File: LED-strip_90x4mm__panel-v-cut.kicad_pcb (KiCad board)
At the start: 2 copper layers, 96 x 90 mm, 912 parts, among them P1 CONN_2, P10 CONN_2, P11 CONN_2, P12 CONN_2, P2 CONN_2, P3 CONN_2, P4 CONN_2, P5 CONN_2, P6 CONN_2, P7 CONN_2, P8 CONN_2, P9 CONN_2

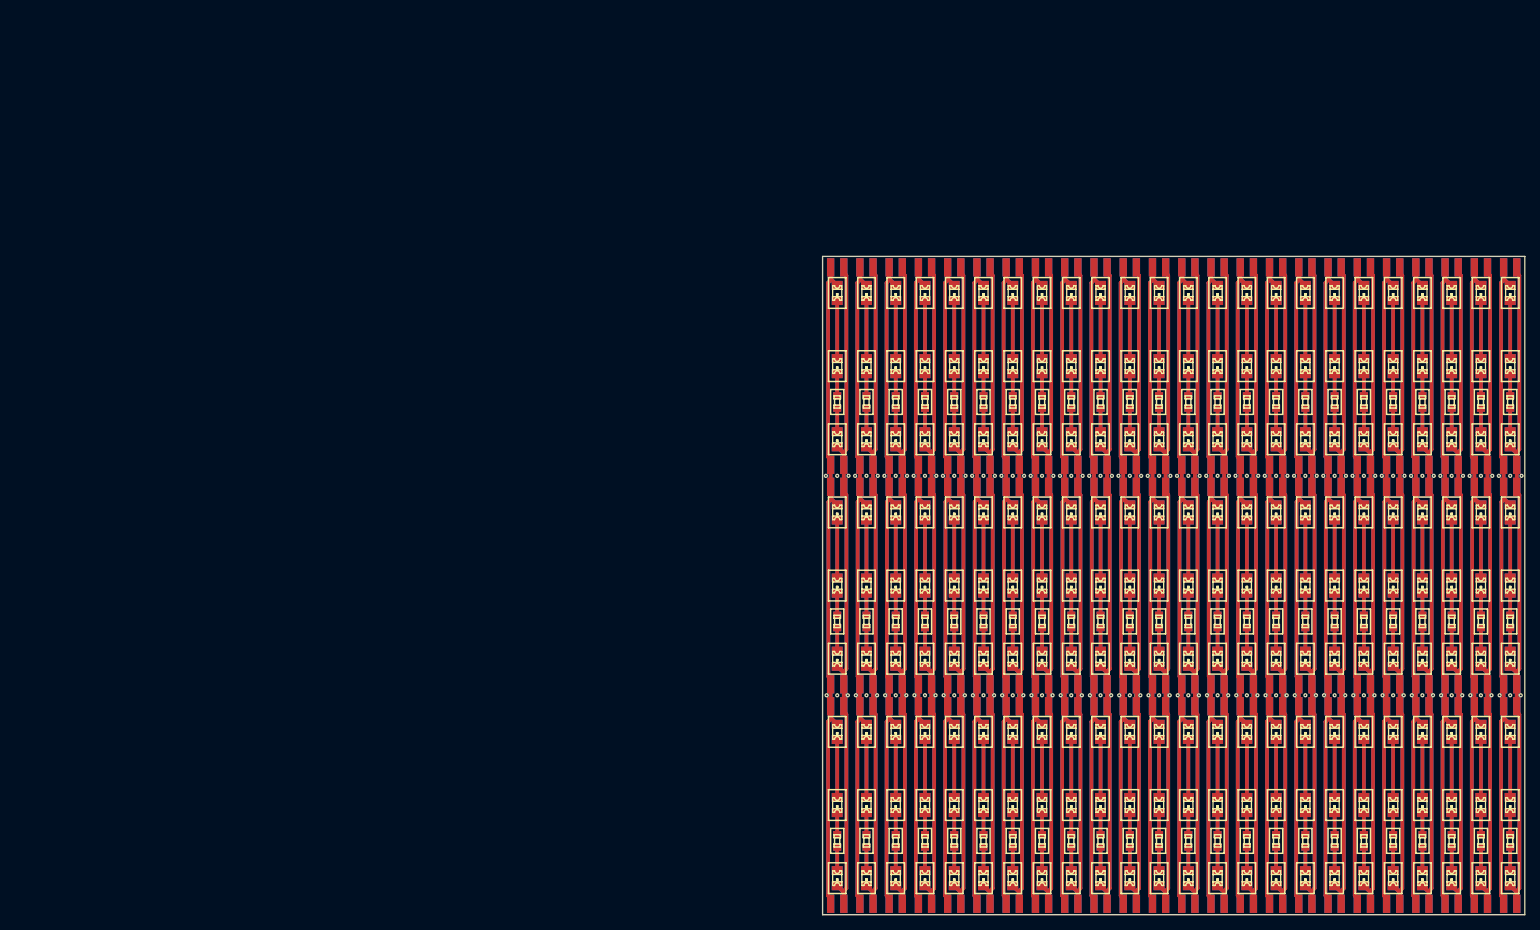
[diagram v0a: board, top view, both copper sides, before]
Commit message: Redid the panel.
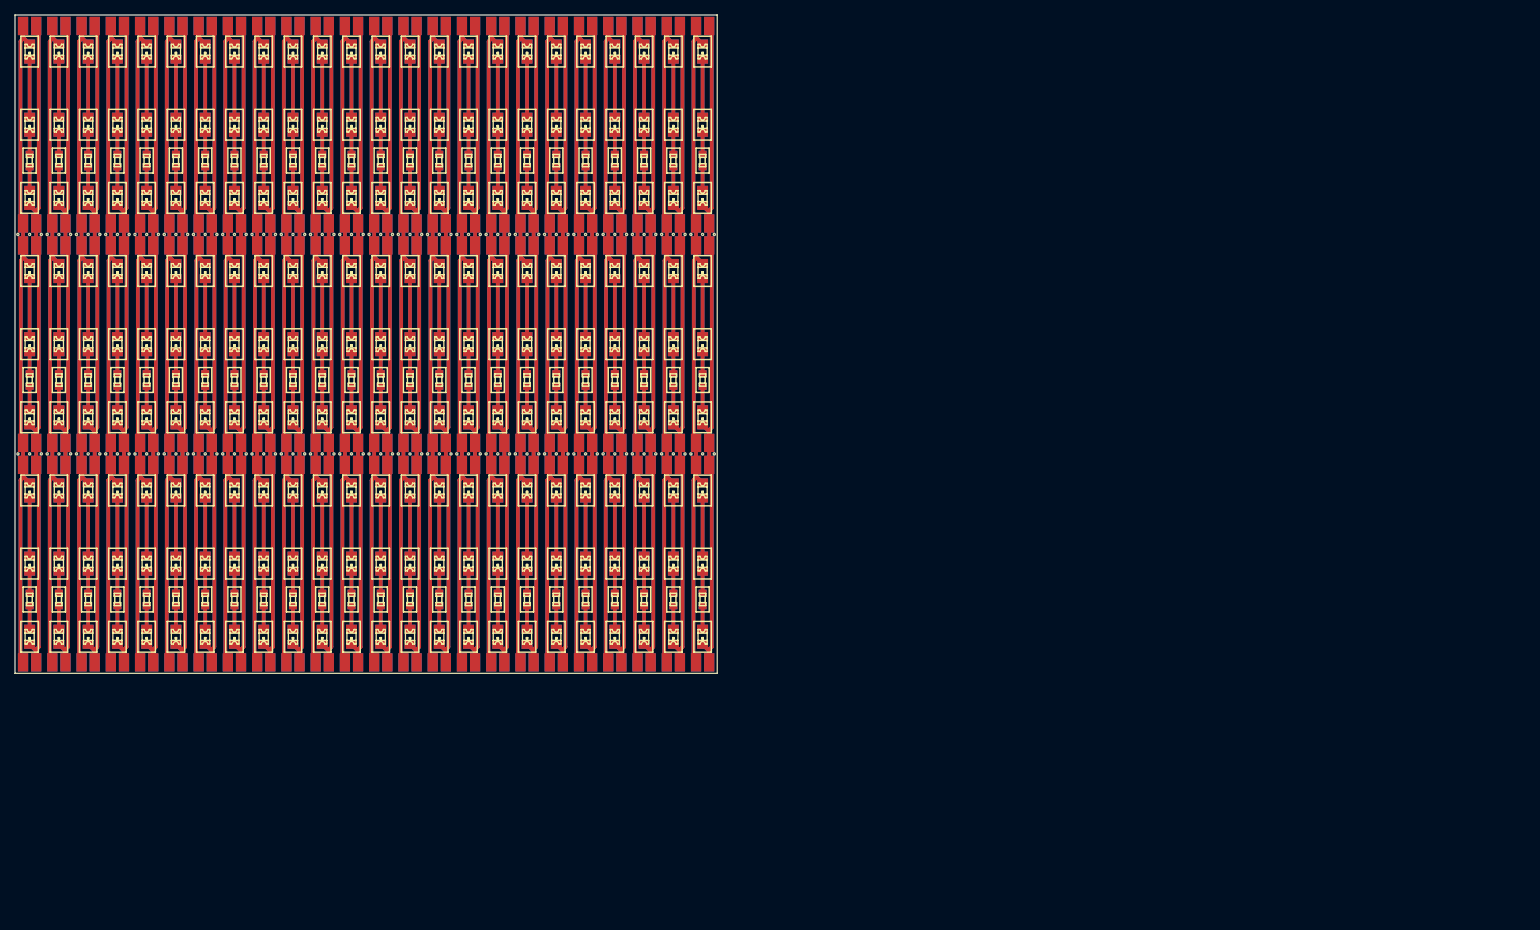
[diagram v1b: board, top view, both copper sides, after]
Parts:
- removed the D1 at (288.5, 153.0)
- removed the D1 at (328.5, 153.0)
- removed the D1 at (312.5, 153.0)
- removed the D1 at (316.5, 153.0)
- removed the D1 at (324.5, 153.0)
- removed the D1 at (320.5, 153.0)
- removed the D1 at (360.5, 153.0)
- removed the D1 at (364.5, 153.0)
- removed the D1 at (356.5, 153.0)
- removed the D1 at (352.5, 153.0)
- removed the D1 at (368.5, 153.0)
- removed the D1 at (284.5, 153.0)
- removed the D1 at (348.5, 153.0)
- removed the D1 at (332.5, 153.0)
- removed the D1 at (336.5, 153.0)
- removed the D1 at (344.5, 153.0)
- removed the D1 at (340.5, 153.0)
- removed the D1 at (372.5, 153.0)
- removed the D1 at (376.5, 153.0)
- removed the D1 at (300.5, 153.0)
- removed the D1 at (304.5, 153.0)
- removed the D1 at (296.5, 153.0)
- removed the D1 at (292.5, 153.0)
- removed the D1 at (308.5, 153.0)
- removed the D10 at (288.5, 93.0)
- removed the D10 at (328.5, 93.0)
- removed the D10 at (312.5, 93.0)
- removed the D10 at (316.5, 93.0)
- removed the D10 at (324.5, 93.0)
- removed the D10 at (320.5, 93.0)
- removed the D10 at (360.5, 93.0)
- removed the D10 at (364.5, 93.0)
- removed the D10 at (356.5, 93.0)
- removed the D10 at (352.5, 93.0)
- removed the D10 at (368.5, 93.0)
- removed the D10 at (284.5, 93.0)
- removed the D10 at (348.5, 93.0)
- removed the D10 at (332.5, 93.0)
- removed the D10 at (336.5, 93.0)
- removed the D10 at (344.5, 93.0)
- removed the D10 at (340.5, 93.0)
- removed the D10 at (372.5, 93.0)
- removed the D10 at (376.5, 93.0)
- removed the D10 at (300.5, 93.0)
- removed the D10 at (304.5, 93.0)
- removed the D10 at (296.5, 93.0)
- removed the D10 at (292.5, 93.0)
- removed the D10 at (308.5, 93.0)
- removed the D11 at (288.5, 103.0)
- removed the D11 at (328.5, 103.0)
- removed the D11 at (312.5, 103.0)
- removed the D11 at (316.5, 103.0)
- removed the D11 at (324.5, 103.0)
- removed the D11 at (320.5, 103.0)
- removed the D11 at (360.5, 103.0)
- removed the D11 at (364.5, 103.0)
- removed the D11 at (356.5, 103.0)
- removed the D11 at (352.5, 103.0)
- removed the D11 at (368.5, 103.0)
- removed the D11 at (284.5, 103.0)
- removed the D11 at (348.5, 103.0)
- removed the D11 at (332.5, 103.0)
- removed the D11 at (336.5, 103.0)
- removed the D11 at (344.5, 103.0)
- removed the D11 at (340.5, 103.0)
- removed the D11 at (372.5, 103.0)
- removed the D11 at (376.5, 103.0)
- removed the D11 at (300.5, 103.0)
- removed the D11 at (304.5, 103.0)
- removed the D11 at (296.5, 103.0)
- removed the D11 at (292.5, 103.0)
- removed the D11 at (308.5, 103.0)
- removed the D12 at (288.5, 113.0)
- removed the D12 at (328.5, 113.0)
- removed the D12 at (312.5, 113.0)
- removed the D12 at (316.5, 113.0)
- removed the D12 at (324.5, 113.0)
- removed the D12 at (320.5, 113.0)
- removed the D12 at (360.5, 113.0)
- removed the D12 at (364.5, 113.0)
- removed the D12 at (356.5, 113.0)
- removed the D12 at (352.5, 113.0)
- removed the D12 at (368.5, 113.0)
- removed the D12 at (284.5, 113.0)
- removed the D12 at (348.5, 113.0)
- removed the D12 at (332.5, 113.0)
- removed the D12 at (336.5, 113.0)
- removed the D12 at (344.5, 113.0)
- removed the D12 at (340.5, 113.0)
- removed the D12 at (372.5, 113.0)
- removed the D12 at (376.5, 113.0)
- removed the D12 at (300.5, 113.0)
- removed the D12 at (304.5, 113.0)
- removed the D12 at (296.5, 113.0)
- removed the D12 at (292.5, 113.0)
- removed the D12 at (308.5, 113.0)
- removed the D13 at (288.5, 123.0)
- removed the D13 at (328.5, 123.0)
- removed the D13 at (312.5, 123.0)
- removed the D13 at (316.5, 123.0)
- removed the D13 at (324.5, 123.0)
- removed the D13 at (320.5, 123.0)
- removed the D13 at (360.5, 123.0)
- removed the D13 at (364.5, 123.0)
- removed the D13 at (356.5, 123.0)
- removed the D13 at (352.5, 123.0)
- removed the D13 at (368.5, 123.0)
- removed the D13 at (284.5, 123.0)
- removed the D13 at (348.5, 123.0)
- removed the D13 at (332.5, 123.0)
- removed the D13 at (336.5, 123.0)
- removed the D13 at (344.5, 123.0)
- removed the D13 at (340.5, 123.0)
- removed the D13 at (372.5, 123.0)
- removed the D13 at (376.5, 123.0)
- removed the D13 at (300.5, 123.0)
- removed the D13 at (304.5, 123.0)
- removed the D13 at (296.5, 123.0)
- removed the D13 at (292.5, 123.0)
- removed the D13 at (308.5, 123.0)
- removed the D14 at (288.5, 133.0)
- removed the D14 at (328.5, 133.0)
- removed the D14 at (312.5, 133.0)
- removed the D14 at (316.5, 133.0)
- removed the D14 at (324.5, 133.0)
- removed the D14 at (320.5, 133.0)
- removed the D14 at (360.5, 133.0)
- removed the D14 at (364.5, 133.0)
- removed the D14 at (356.5, 133.0)
- removed the D14 at (352.5, 133.0)
- removed the D14 at (368.5, 133.0)
- removed the D14 at (284.5, 133.0)
- removed the D14 at (348.5, 133.0)
- removed the D14 at (332.5, 133.0)
- removed the D14 at (336.5, 133.0)
- removed the D14 at (344.5, 133.0)
- removed the D14 at (340.5, 133.0)
- removed the D14 at (372.5, 133.0)
- removed the D14 at (376.5, 133.0)
- removed the D14 at (300.5, 133.0)
- removed the D14 at (304.5, 133.0)
- removed the D14 at (296.5, 133.0)
- removed the D14 at (292.5, 133.0)
- removed the D14 at (308.5, 133.0)
- removed the D15 at (288.5, 143.0)
- removed the D15 at (328.5, 143.0)
- removed the D15 at (312.5, 143.0)
- removed the D15 at (316.5, 143.0)
- removed the D15 at (324.5, 143.0)
- removed the D15 at (320.5, 143.0)
- removed the D15 at (360.5, 143.0)
- removed the D15 at (364.5, 143.0)
- removed the D15 at (356.5, 143.0)
- removed the D15 at (352.5, 143.0)
- removed the D15 at (368.5, 143.0)
- removed the D15 at (284.5, 143.0)
- removed the D15 at (348.5, 143.0)
- removed the D15 at (332.5, 143.0)
- removed the D15 at (336.5, 143.0)
- removed the D15 at (344.5, 143.0)
- removed the D15 at (340.5, 143.0)
- removed the D15 at (372.5, 143.0)
- removed the D15 at (376.5, 143.0)
- removed the D15 at (300.5, 143.0)
- removed the D15 at (304.5, 143.0)
- removed the D15 at (296.5, 143.0)
- removed the D15 at (292.5, 143.0)
- removed the D15 at (308.5, 143.0)
- removed the D16 at (288.5, 153.0)
- removed the D16 at (328.5, 153.0)
- removed the D16 at (312.5, 153.0)
- removed the D16 at (316.5, 153.0)
- removed the D16 at (324.5, 153.0)
- removed the D16 at (320.5, 153.0)
- removed the D16 at (360.5, 153.0)
- removed the D16 at (364.5, 153.0)
- removed the D16 at (356.5, 153.0)
- removed the D16 at (352.5, 153.0)
- removed the D16 at (368.5, 153.0)
- removed the D16 at (284.5, 153.0)
- removed the D16 at (348.5, 153.0)
- removed the D16 at (332.5, 153.0)
- removed the D16 at (336.5, 153.0)
- removed the D16 at (344.5, 153.0)
- removed the D16 at (340.5, 153.0)
- removed the D16 at (372.5, 153.0)
- removed the D16 at (376.5, 153.0)
- removed the D16 at (300.5, 153.0)
- removed the D16 at (304.5, 153.0)
- removed the D16 at (296.5, 153.0)
- removed the D16 at (292.5, 153.0)
- removed the D16 at (308.5, 153.0)
- removed the D17 at (288.5, 163.0)
- removed the D17 at (328.5, 163.0)
- removed the D17 at (312.5, 163.0)
- removed the D17 at (316.5, 163.0)
- removed the D17 at (324.5, 163.0)
- removed the D17 at (320.5, 163.0)
- removed the D17 at (360.5, 163.0)
- removed the D17 at (364.5, 163.0)
- removed the D17 at (356.5, 163.0)
- removed the D17 at (352.5, 163.0)
- removed the D17 at (368.5, 163.0)
- removed the D17 at (284.5, 163.0)
- removed the D17 at (348.5, 163.0)
- removed the D17 at (332.5, 163.0)
- removed the D17 at (336.5, 163.0)
- removed the D17 at (344.5, 163.0)
- removed the D17 at (340.5, 163.0)
- removed the D17 at (372.5, 163.0)
- removed the D17 at (376.5, 163.0)
- removed the D17 at (300.5, 163.0)
- removed the D17 at (304.5, 163.0)
- removed the D17 at (296.5, 163.0)
- removed the D17 at (292.5, 163.0)
- removed the D17 at (308.5, 163.0)
- removed the D18 at (288.5, 173.0)
- removed the D18 at (328.5, 173.0)
- removed the D18 at (312.5, 173.0)
- removed the D18 at (316.5, 173.0)
- removed the D18 at (324.5, 173.0)
- removed the D18 at (320.5, 173.0)
- removed the D18 at (360.5, 173.0)
- removed the D18 at (364.5, 173.0)
- removed the D18 at (356.5, 173.0)
- removed the D18 at (352.5, 173.0)
- removed the D18 at (368.5, 173.0)
- removed the D18 at (284.5, 173.0)
- removed the D18 at (348.5, 173.0)
- removed the D18 at (332.5, 173.0)
- removed the D18 at (336.5, 173.0)
- removed the D18 at (344.5, 173.0)
- removed the D18 at (340.5, 173.0)
- removed the D18 at (372.5, 173.0)
- removed the D18 at (376.5, 173.0)
- removed the D18 at (300.5, 173.0)
- removed the D18 at (304.5, 173.0)
- removed the D18 at (296.5, 173.0)
- removed the D18 at (292.5, 173.0)
- removed the D18 at (308.5, 173.0)
- removed the D2 at (288.5, 163.0)
- removed the D2 at (328.5, 163.0)
- removed the D2 at (312.5, 163.0)
- removed the D2 at (316.5, 163.0)
- removed the D2 at (324.5, 163.0)
- removed the D2 at (320.5, 163.0)
- removed the D2 at (360.5, 163.0)
- removed the D2 at (364.5, 163.0)
- removed the D2 at (356.5, 163.0)
- removed the D2 at (352.5, 163.0)
- removed the D2 at (368.5, 163.0)
- removed the D2 at (284.5, 163.0)
- removed the D2 at (348.5, 163.0)
- removed the D2 at (332.5, 163.0)
- removed the D2 at (336.5, 163.0)
- removed the D2 at (344.5, 163.0)
- removed the D2 at (340.5, 163.0)
- removed the D2 at (372.5, 163.0)
- removed the D2 at (376.5, 163.0)
- removed the D2 at (300.5, 163.0)
- removed the D2 at (304.5, 163.0)
- removed the D2 at (296.5, 163.0)
- removed the D2 at (292.5, 163.0)
- removed the D2 at (308.5, 163.0)
- removed the D3 at (288.5, 173.0)
- removed the D3 at (328.5, 173.0)
- removed the D3 at (312.5, 173.0)
- removed the D3 at (316.5, 173.0)
- removed the D3 at (324.5, 173.0)
- removed the D3 at (320.5, 173.0)
- removed the D3 at (360.5, 173.0)
- removed the D3 at (364.5, 173.0)
- removed the D3 at (356.5, 173.0)
- removed the D3 at (352.5, 173.0)
- removed the D3 at (368.5, 173.0)
- removed the D3 at (284.5, 173.0)
- removed the D3 at (348.5, 173.0)
- removed the D3 at (332.5, 173.0)
- removed the D3 at (336.5, 173.0)
- removed the D3 at (344.5, 173.0)
- removed the D3 at (340.5, 173.0)
- removed the D3 at (372.5, 173.0)
- removed the D3 at (376.5, 173.0)
- removed the D3 at (300.5, 173.0)
- removed the D3 at (304.5, 173.0)
- removed the D3 at (296.5, 173.0)
- removed the D3 at (292.5, 173.0)
- removed the D3 at (308.5, 173.0)
- removed the D4 at (288.5, 123.0)
- removed the D4 at (328.5, 123.0)
- removed the D4 at (312.5, 123.0)
- removed the D4 at (316.5, 123.0)
- removed the D4 at (324.5, 123.0)
- removed the D4 at (320.5, 123.0)
- removed the D4 at (360.5, 123.0)
- removed the D4 at (364.5, 123.0)
- removed the D4 at (356.5, 123.0)
- removed the D4 at (352.5, 123.0)
- removed the D4 at (368.5, 123.0)
- removed the D4 at (284.5, 123.0)
- removed the D4 at (348.5, 123.0)
- removed the D4 at (332.5, 123.0)
- removed the D4 at (336.5, 123.0)
- removed the D4 at (344.5, 123.0)
- removed the D4 at (340.5, 123.0)
- removed the D4 at (372.5, 123.0)
- removed the D4 at (376.5, 123.0)
- removed the D4 at (300.5, 123.0)
- removed the D4 at (304.5, 123.0)
- removed the D4 at (296.5, 123.0)
- removed the D4 at (292.5, 123.0)
- removed the D4 at (308.5, 123.0)
- removed the D5 at (288.5, 133.0)
- removed the D5 at (328.5, 133.0)
- removed the D5 at (312.5, 133.0)
- removed the D5 at (316.5, 133.0)
- removed the D5 at (324.5, 133.0)
- removed the D5 at (320.5, 133.0)
- removed the D5 at (360.5, 133.0)
- removed the D5 at (364.5, 133.0)
- removed the D5 at (356.5, 133.0)
- removed the D5 at (352.5, 133.0)
- removed the D5 at (368.5, 133.0)
- removed the D5 at (284.5, 133.0)
- removed the D5 at (348.5, 133.0)
- removed the D5 at (332.5, 133.0)
- removed the D5 at (336.5, 133.0)
- removed the D5 at (344.5, 133.0)
- removed the D5 at (340.5, 133.0)
- removed the D5 at (372.5, 133.0)
- removed the D5 at (376.5, 133.0)
- removed the D5 at (300.5, 133.0)
- removed the D5 at (304.5, 133.0)
- removed the D5 at (296.5, 133.0)
- removed the D5 at (292.5, 133.0)
- removed the D5 at (308.5, 133.0)
- removed the D6 at (288.5, 143.0)
- removed the D6 at (328.5, 143.0)
- removed the D6 at (312.5, 143.0)
- removed the D6 at (316.5, 143.0)
- removed the D6 at (324.5, 143.0)
- removed the D6 at (320.5, 143.0)
- removed the D6 at (360.5, 143.0)
- removed the D6 at (364.5, 143.0)
- removed the D6 at (356.5, 143.0)
- removed the D6 at (352.5, 143.0)
- removed the D6 at (368.5, 143.0)
- removed the D6 at (284.5, 143.0)
- removed the D6 at (348.5, 143.0)
- removed the D6 at (332.5, 143.0)
- removed the D6 at (336.5, 143.0)
- removed the D6 at (344.5, 143.0)
- removed the D6 at (340.5, 143.0)
- removed the D6 at (372.5, 143.0)
- removed the D6 at (376.5, 143.0)
- removed the D6 at (300.5, 143.0)
- removed the D6 at (304.5, 143.0)
- removed the D6 at (296.5, 143.0)
- removed the D6 at (292.5, 143.0)
- removed the D6 at (308.5, 143.0)
- removed the D7 at (288.5, 93.0)
- removed the D7 at (328.5, 93.0)
- removed the D7 at (312.5, 93.0)
- removed the D7 at (316.5, 93.0)
- removed the D7 at (324.5, 93.0)
- removed the D7 at (320.5, 93.0)
- removed the D7 at (360.5, 93.0)
- removed the D7 at (364.5, 93.0)
- removed the D7 at (356.5, 93.0)
- removed the D7 at (352.5, 93.0)
- removed the D7 at (368.5, 93.0)
- removed the D7 at (284.5, 93.0)
- removed the D7 at (348.5, 93.0)
- removed the D7 at (332.5, 93.0)
- removed the D7 at (336.5, 93.0)
- removed the D7 at (344.5, 93.0)
- removed the D7 at (340.5, 93.0)
- removed the D7 at (372.5, 93.0)
- removed the D7 at (376.5, 93.0)
- removed the D7 at (300.5, 93.0)
- removed the D7 at (304.5, 93.0)
- removed the D7 at (296.5, 93.0)
- removed the D7 at (292.5, 93.0)
- removed the D7 at (308.5, 93.0)
- removed the D8 at (288.5, 103.0)
- removed the D8 at (328.5, 103.0)
- removed the D8 at (312.5, 103.0)
- removed the D8 at (316.5, 103.0)
- removed the D8 at (324.5, 103.0)
- removed the D8 at (320.5, 103.0)
- removed the D8 at (360.5, 103.0)
- removed the D8 at (364.5, 103.0)
- removed the D8 at (356.5, 103.0)
- removed the D8 at (352.5, 103.0)
- removed the D8 at (368.5, 103.0)
- removed the D8 at (284.5, 103.0)
- removed the D8 at (348.5, 103.0)
- removed the D8 at (332.5, 103.0)
- removed the D8 at (336.5, 103.0)
- removed the D8 at (344.5, 103.0)
- removed the D8 at (340.5, 103.0)
- removed the D8 at (372.5, 103.0)
- removed the D8 at (376.5, 103.0)
- removed the D8 at (300.5, 103.0)
- removed the D8 at (304.5, 103.0)
- removed the D8 at (296.5, 103.0)
- removed the D8 at (292.5, 103.0)
- removed the D8 at (308.5, 103.0)
- removed the D9 at (288.5, 113.0)
- removed the D9 at (328.5, 113.0)
- removed the D9 at (312.5, 113.0)
- removed the D9 at (316.5, 113.0)
- removed the D9 at (324.5, 113.0)
- removed the D9 at (320.5, 113.0)
- removed the D9 at (360.5, 113.0)
- removed the D9 at (364.5, 113.0)
- removed the D9 at (356.5, 113.0)
- removed the D9 at (352.5, 113.0)
- removed the D9 at (368.5, 113.0)
- removed the D9 at (284.5, 113.0)
- removed the D9 at (348.5, 113.0)
- removed the D9 at (332.5, 113.0)
- removed the D9 at (336.5, 113.0)
- removed the D9 at (344.5, 113.0)
- removed the D9 at (340.5, 113.0)
- removed the D9 at (372.5, 113.0)
- removed the D9 at (376.5, 113.0)
- removed the D9 at (300.5, 113.0)
- removed the D9 at (304.5, 113.0)
- removed the D9 at (296.5, 113.0)
- removed the D9 at (292.5, 113.0)
- removed the D9 at (308.5, 113.0)
- removed the G1 at (288.6, 98.1)
- removed the G1 at (328.6, 98.1)
- removed the G1 at (312.6, 98.1)
- removed the G1 at (316.6, 98.1)
- removed the G1 at (324.6, 98.1)
- removed the G1 at (320.6, 98.1)
- removed the G1 at (360.6, 98.1)
- removed the G1 at (364.6, 98.1)
- removed the G1 at (356.6, 98.1)
- removed the G1 at (352.6, 98.1)
- removed the G1 at (368.6, 98.1)
- removed the G1 at (284.6, 98.1)
- removed the G1 at (348.6, 98.1)
- removed the G1 at (332.6, 98.1)
- removed the G1 at (336.6, 98.1)
- removed the G1 at (344.6, 98.1)
- removed the G1 at (340.6, 98.1)
- removed the G1 at (372.6, 98.1)
- removed the G1 at (376.6, 98.1)
- removed the G1 at (300.6, 98.1)
- removed the G1 at (304.6, 98.1)
- removed the G1 at (296.6, 98.1)
- removed the G1 at (292.6, 98.1)
- removed the G1 at (308.6, 98.1)
- removed the G2 at (288.5, 128.1)
- removed the G2 at (328.5, 128.1)
- removed the G2 at (312.5, 128.1)
- removed the G2 at (316.5, 128.1)
- removed the G2 at (324.5, 128.1)
- removed the G2 at (320.5, 128.1)
- removed the G2 at (360.5, 128.1)
- removed the G2 at (364.5, 128.1)
- removed the G2 at (356.5, 128.1)
- removed the G2 at (352.5, 128.1)
- removed the G2 at (368.5, 128.1)
- removed the G2 at (284.5, 128.1)
- removed the G2 at (348.5, 128.1)
- removed the G2 at (332.5, 128.1)
- removed the G2 at (336.5, 128.1)
- removed the G2 at (344.5, 128.1)
- removed the G2 at (340.5, 128.1)
- removed the G2 at (372.5, 128.1)
- removed the G2 at (376.5, 128.1)
- removed the G2 at (300.5, 128.1)
- removed the G2 at (304.5, 128.1)
- removed the G2 at (296.5, 128.1)
- removed the G2 at (292.5, 128.1)
- removed the G2 at (308.5, 128.1)
- removed the P1 at (288.5, 176.5)
- removed the P1 at (328.5, 176.5)
- removed the P1 at (312.5, 176.5)
- removed the P1 at (316.5, 176.5)
- removed the P1 at (324.5, 176.5)
- removed the P1 at (320.5, 176.5)
- removed the P1 at (360.5, 176.5)
- removed the P1 at (364.5, 176.5)
- removed the P1 at (356.5, 176.5)
- removed the P1 at (352.5, 176.5)
- removed the P1 at (368.5, 176.5)
- removed the P1 at (284.5, 176.5)
- removed the P1 at (348.5, 176.5)
- removed the P1 at (332.5, 176.5)
- removed the P1 at (336.5, 176.5)
- removed the P1 at (344.5, 176.5)
- removed the P1 at (340.5, 176.5)
- removed the P1 at (372.5, 176.5)
- removed the P1 at (376.5, 176.5)
- removed the P1 at (300.5, 176.5)
- removed the P1 at (304.5, 176.5)
- removed the P1 at (296.5, 176.5)
- removed the P1 at (292.5, 176.5)
- removed the P1 at (308.5, 176.5)
- removed the P10 at (288.5, 146.5)
- removed the P10 at (328.5, 146.5)
- removed the P10 at (312.5, 146.5)
- removed the P10 at (316.5, 146.5)
- removed the P10 at (324.5, 146.5)
- removed the P10 at (320.5, 146.5)
- removed the P10 at (360.5, 146.5)
- removed the P10 at (364.5, 146.5)
- removed the P10 at (356.5, 146.5)
- removed the P10 at (352.5, 146.5)
- removed the P10 at (368.5, 146.5)
- removed the P10 at (284.5, 146.5)
- removed the P10 at (348.5, 146.5)
- removed the P10 at (332.5, 146.5)
- removed the P10 at (336.5, 146.5)
- removed the P10 at (344.5, 146.5)
- removed the P10 at (340.5, 146.5)
- removed the P10 at (372.5, 146.5)
- removed the P10 at (376.5, 146.5)
- removed the P10 at (300.5, 146.5)
- removed the P10 at (304.5, 146.5)
- removed the P10 at (296.5, 146.5)
- removed the P10 at (292.5, 146.5)
- removed the P10 at (308.5, 146.5)
- removed the P11 at (288.5, 149.5)
- removed the P11 at (328.5, 149.5)
- removed the P11 at (312.5, 149.5)
- removed the P11 at (316.5, 149.5)
- removed the P11 at (324.5, 149.5)
- removed the P11 at (320.5, 149.5)
- removed the P11 at (360.5, 149.5)
- removed the P11 at (364.5, 149.5)
- removed the P11 at (356.5, 149.5)
- removed the P11 at (352.5, 149.5)
- removed the P11 at (368.5, 149.5)
- removed the P11 at (284.5, 149.5)
- removed the P11 at (348.5, 149.5)
- removed the P11 at (332.5, 149.5)
- removed the P11 at (336.5, 149.5)
- removed the P11 at (344.5, 149.5)
- removed the P11 at (340.5, 149.5)
- removed the P11 at (372.5, 149.5)
- removed the P11 at (376.5, 149.5)
- removed the P11 at (300.5, 149.5)
- removed the P11 at (304.5, 149.5)
- removed the P11 at (296.5, 149.5)
- removed the P11 at (292.5, 149.5)
- removed the P11 at (308.5, 149.5)
- removed the P12 at (288.5, 176.5)
- removed the P12 at (328.5, 176.5)
- removed the P12 at (312.5, 176.5)
- removed the P12 at (316.5, 176.5)
- removed the P12 at (324.5, 176.5)
- removed the P12 at (320.5, 176.5)
- removed the P12 at (360.5, 176.5)
- removed the P12 at (364.5, 176.5)
- removed the P12 at (356.5, 176.5)
- removed the P12 at (352.5, 176.5)
- removed the P12 at (368.5, 176.5)
- removed the P12 at (284.5, 176.5)
- removed the P12 at (348.5, 176.5)
- removed the P12 at (332.5, 176.5)
- removed the P12 at (336.5, 176.5)
- removed the P12 at (344.5, 176.5)
- removed the P12 at (340.5, 176.5)
- removed the P12 at (372.5, 176.5)
- removed the P12 at (376.5, 176.5)
- removed the P12 at (300.5, 176.5)
- removed the P12 at (304.5, 176.5)
- removed the P12 at (296.5, 176.5)
- removed the P12 at (292.5, 176.5)
- removed the P12 at (308.5, 176.5)
- removed the P2 at (288.5, 149.5)
- removed the P2 at (348.5, 149.5)
- removed the P2 at (344.5, 149.5)
- removed the P2 at (340.5, 149.5)
- removed the P2 at (336.5, 149.5)
- removed the P2 at (332.5, 149.5)
- removed the P2 at (328.5, 149.5)
- removed the P2 at (324.5, 149.5)
- removed the P2 at (320.5, 149.5)
- removed the P2 at (316.5, 149.5)
- removed the P2 at (312.5, 149.5)
- removed the P2 at (284.5, 149.5)
- removed the P2 at (308.5, 149.5)
- removed the P2 at (304.5, 149.5)
- removed the P2 at (300.5, 149.5)
- removed the P2 at (296.5, 149.5)
- removed the P2 at (292.5, 149.5)
- removed the P2 at (372.5, 149.5)
- removed the P2 at (376.5, 149.5)
- removed the P2 at (368.5, 149.5)
- removed the P2 at (364.5, 149.5)
- removed the P2 at (360.5, 149.5)
- removed the P2 at (356.5, 149.5)
- removed the P2 at (352.5, 149.5)
- removed the P3 at (288.5, 146.5)
- removed the P3 at (328.5, 146.5)
- removed the P3 at (312.5, 146.5)
- removed the P3 at (316.5, 146.5)
- removed the P3 at (324.5, 146.5)
- removed the P3 at (320.5, 146.5)
- removed the P3 at (360.5, 146.5)
- removed the P3 at (364.5, 146.5)
- removed the P3 at (356.5, 146.5)
- removed the P3 at (352.5, 146.5)
- removed the P3 at (368.5, 146.5)
- removed the P3 at (284.5, 146.5)
- removed the P3 at (348.5, 146.5)
- removed the P3 at (332.5, 146.5)
- removed the P3 at (336.5, 146.5)
- removed the P3 at (344.5, 146.5)
- removed the P3 at (340.5, 146.5)
- removed the P3 at (372.5, 146.5)
- removed the P3 at (376.5, 146.5)
- removed the P3 at (300.5, 146.5)
- removed the P3 at (304.5, 146.5)
- removed the P3 at (296.5, 146.5)
- removed the P3 at (292.5, 146.5)
- removed the P3 at (308.5, 146.5)
- removed the P4 at (288.5, 119.5)
- removed the P4 at (348.5, 119.5)
- removed the P4 at (344.5, 119.5)
- removed the P4 at (340.5, 119.5)
- removed the P4 at (336.5, 119.5)
- removed the P4 at (332.5, 119.5)
- removed the P4 at (328.5, 119.5)
- removed the P4 at (324.5, 119.5)
- removed the P4 at (320.5, 119.5)
- removed the P4 at (316.5, 119.5)
- removed the P4 at (312.5, 119.5)
- removed the P4 at (284.5, 119.5)
- removed the P4 at (308.5, 119.5)
- removed the P4 at (304.5, 119.5)
- removed the P4 at (300.5, 119.5)
- removed the P4 at (296.5, 119.5)
- removed the P4 at (292.5, 119.5)
- removed the P4 at (372.5, 119.5)
- removed the P4 at (376.5, 119.5)
- removed the P4 at (368.5, 119.5)
- removed the P4 at (364.5, 119.5)
- removed the P4 at (360.5, 119.5)
- removed the P4 at (356.5, 119.5)
- removed the P4 at (352.5, 119.5)
- removed the P5 at (288.5, 116.5)
- removed the P5 at (328.5, 116.5)
- removed the P5 at (312.5, 116.5)
- removed the P5 at (316.5, 116.5)
- removed the P5 at (324.5, 116.5)
- removed the P5 at (320.5, 116.5)
- removed the P5 at (360.5, 116.5)
- removed the P5 at (364.5, 116.5)
- removed the P5 at (356.5, 116.5)
- removed the P5 at (352.5, 116.5)
- removed the P5 at (368.5, 116.5)
- removed the P5 at (284.5, 116.5)
- removed the P5 at (348.5, 116.5)
- removed the P5 at (332.5, 116.5)
- removed the P5 at (336.5, 116.5)
- removed the P5 at (344.5, 116.5)
- removed the P5 at (340.5, 116.5)
- removed the P5 at (372.5, 116.5)
- removed the P5 at (376.5, 116.5)
- removed the P5 at (300.5, 116.5)
- removed the P5 at (304.5, 116.5)
- removed the P5 at (296.5, 116.5)
- removed the P5 at (292.5, 116.5)
- removed the P5 at (308.5, 116.5)
- removed the P6 at (288.5, 89.5)
- removed the P6 at (328.5, 89.5)
- removed the P6 at (312.5, 89.5)
- removed the P6 at (316.5, 89.5)
- removed the P6 at (324.5, 89.5)
- removed the P6 at (320.5, 89.5)
- removed the P6 at (360.5, 89.5)
- removed the P6 at (364.5, 89.5)
- removed the P6 at (356.5, 89.5)
- removed the P6 at (352.5, 89.5)
- removed the P6 at (368.5, 89.5)
- removed the P6 at (284.5, 89.5)
- removed the P6 at (348.5, 89.5)
- removed the P6 at (332.5, 89.5)
- removed the P6 at (336.5, 89.5)
- removed the P6 at (344.5, 89.5)
- removed the P6 at (340.5, 89.5)
- removed the P6 at (372.5, 89.5)
- removed the P6 at (376.5, 89.5)
- removed the P6 at (300.5, 89.5)
- removed the P6 at (304.5, 89.5)
- removed the P6 at (296.5, 89.5)
- removed the P6 at (292.5, 89.5)
- removed the P6 at (308.5, 89.5)
- removed the P7 at (288.5, 89.5)
- removed the P7 at (328.5, 89.5)
- removed the P7 at (312.5, 89.5)
- removed the P7 at (316.5, 89.5)
- removed the P7 at (324.5, 89.5)
- removed the P7 at (320.5, 89.5)
- removed the P7 at (360.5, 89.5)
- removed the P7 at (364.5, 89.5)
- removed the P7 at (356.5, 89.5)
- removed the P7 at (352.5, 89.5)
- removed the P7 at (368.5, 89.5)
- removed the P7 at (284.5, 89.5)
- removed the P7 at (348.5, 89.5)
- removed the P7 at (332.5, 89.5)
- removed the P7 at (336.5, 89.5)
- removed the P7 at (344.5, 89.5)
- removed the P7 at (340.5, 89.5)
- removed the P7 at (372.5, 89.5)
- removed the P7 at (376.5, 89.5)
- removed the P7 at (300.5, 89.5)
- removed the P7 at (304.5, 89.5)
- removed the P7 at (296.5, 89.5)
- removed the P7 at (292.5, 89.5)
- removed the P7 at (308.5, 89.5)
- removed the P8 at (288.5, 116.5)
- removed the P8 at (328.5, 116.5)
- removed the P8 at (312.5, 116.5)
- removed the P8 at (316.5, 116.5)
- removed the P8 at (324.5, 116.5)
- removed the P8 at (320.5, 116.5)
- removed the P8 at (360.5, 116.5)
- removed the P8 at (364.5, 116.5)
- removed the P8 at (356.5, 116.5)
- removed the P8 at (352.5, 116.5)
- removed the P8 at (368.5, 116.5)
- removed the P8 at (284.5, 116.5)
- removed the P8 at (348.5, 116.5)
- removed the P8 at (332.5, 116.5)
- removed the P8 at (336.5, 116.5)
- removed the P8 at (344.5, 116.5)
- removed the P8 at (340.5, 116.5)
- removed the P8 at (372.5, 116.5)
- removed the P8 at (376.5, 116.5)
- removed the P8 at (300.5, 116.5)
- removed the P8 at (304.5, 116.5)
- removed the P8 at (296.5, 116.5)
- removed the P8 at (292.5, 116.5)
- removed the P8 at (308.5, 116.5)
- removed the P9 at (288.5, 119.5)
- removed the P9 at (328.5, 119.5)
- removed the P9 at (312.5, 119.5)
- removed the P9 at (316.5, 119.5)
- removed the P9 at (324.5, 119.5)
- removed the P9 at (320.5, 119.5)
- removed the P9 at (360.5, 119.5)
- removed the P9 at (364.5, 119.5)
- removed the P9 at (356.5, 119.5)
- removed the P9 at (352.5, 119.5)
- removed the P9 at (368.5, 119.5)
- removed the P9 at (284.5, 119.5)
- removed the P9 at (348.5, 119.5)
- removed the P9 at (332.5, 119.5)
- removed the P9 at (336.5, 119.5)
- removed the P9 at (344.5, 119.5)
- removed the P9 at (340.5, 119.5)
- removed the P9 at (372.5, 119.5)
- removed the P9 at (376.5, 119.5)
- removed the P9 at (300.5, 119.5)
- removed the P9 at (304.5, 119.5)
- removed the P9 at (296.5, 119.5)
- removed the P9 at (292.5, 119.5)
- removed the P9 at (308.5, 119.5)
- removed the R1 at (288.5, 167.9)
- removed the R1 at (328.5, 167.9)
- removed the R1 at (312.5, 167.9)
- removed the R1 at (316.5, 167.9)
- removed the R1 at (324.5, 167.9)
- removed the R1 at (320.5, 167.9)
- removed the R1 at (360.5, 167.9)
- removed the R1 at (364.5, 167.9)
- removed the R1 at (356.5, 167.9)
- removed the R1 at (352.5, 167.9)
- removed the R1 at (368.5, 167.9)
- removed the R1 at (284.5, 167.9)
- removed the R1 at (348.5, 167.9)
- removed the R1 at (332.5, 167.9)
- removed the R1 at (336.5, 167.9)
- removed the R1 at (344.5, 167.9)
- removed the R1 at (340.5, 167.9)
- removed the R1 at (372.5, 167.9)
- removed the R1 at (376.5, 167.9)
- removed the R1 at (300.5, 167.9)
- removed the R1 at (304.5, 167.9)
- removed the R1 at (296.5, 167.9)
- removed the R1 at (292.5, 167.9)
- removed the R1 at (308.5, 167.9)
- removed the R2 at (288.5, 137.9)
- removed the R2 at (328.5, 137.9)
- removed the R2 at (312.5, 137.9)
- removed the R2 at (316.5, 137.9)
- removed the R2 at (324.5, 137.9)
- removed the R2 at (320.5, 137.9)
- removed the R2 at (360.5, 137.9)
- removed the R2 at (364.5, 137.9)
- removed the R2 at (356.5, 137.9)
- removed the R2 at (352.5, 137.9)
- removed the R2 at (368.5, 137.9)
- removed the R2 at (284.5, 137.9)
- removed the R2 at (348.5, 137.9)
- removed the R2 at (332.5, 137.9)
- removed the R2 at (336.5, 137.9)
- removed the R2 at (344.5, 137.9)
- removed the R2 at (340.5, 137.9)
- removed the R2 at (372.5, 137.9)
- removed the R2 at (376.5, 137.9)
- removed the R2 at (300.5, 137.9)
- removed the R2 at (304.5, 137.9)
- removed the R2 at (296.5, 137.9)
- removed the R2 at (292.5, 137.9)
- removed the R2 at (308.5, 137.9)
- removed the R3 at (288.5, 107.9)
- removed the R3 at (328.5, 107.9)
- removed the R3 at (312.5, 107.9)
- removed the R3 at (316.5, 107.9)
- removed the R3 at (324.5, 107.9)
- removed the R3 at (320.5, 107.9)
- removed the R3 at (360.5, 107.9)
- removed the R3 at (364.5, 107.9)
- removed the R3 at (356.5, 107.9)
- removed the R3 at (352.5, 107.9)
- removed the R3 at (368.5, 107.9)
- removed the R3 at (284.5, 107.9)
- removed the R3 at (348.5, 107.9)
- removed the R3 at (332.5, 107.9)
- removed the R3 at (336.5, 107.9)
- removed the R3 at (344.5, 107.9)
- removed the R3 at (340.5, 107.9)
- removed the R3 at (372.5, 107.9)
- removed the R3 at (376.5, 107.9)
- removed the R3 at (300.5, 107.9)
- removed the R3 at (304.5, 107.9)
- removed the R3 at (296.5, 107.9)
- removed the R3 at (292.5, 107.9)
- removed the R3 at (308.5, 107.9)
- removed the R4 at (288.5, 107.9)
- removed the R4 at (328.5, 107.9)
- removed the R4 at (312.5, 107.9)
- removed the R4 at (316.5, 107.9)
- removed the R4 at (324.5, 107.9)
- removed the R4 at (320.5, 107.9)
- removed the R4 at (360.5, 107.9)
- removed the R4 at (364.5, 107.9)
- removed the R4 at (356.5, 107.9)
- removed the R4 at (352.5, 107.9)
- removed the R4 at (368.5, 107.9)
- removed the R4 at (284.5, 107.9)
- removed the R4 at (348.5, 107.9)
- removed the R4 at (332.5, 107.9)
- removed the R4 at (336.5, 107.9)
- removed the R4 at (344.5, 107.9)
- removed the R4 at (340.5, 107.9)
- removed the R4 at (372.5, 107.9)
- removed the R4 at (376.5, 107.9)
- removed the R4 at (300.5, 107.9)
- removed the R4 at (304.5, 107.9)
- removed the R4 at (296.5, 107.9)
- removed the R4 at (292.5, 107.9)
- removed the R4 at (308.5, 107.9)
- removed the R5 at (288.5, 137.9)
- removed the R5 at (328.5, 137.9)
- removed the R5 at (312.5, 137.9)
- removed the R5 at (316.5, 137.9)
- removed the R5 at (324.5, 137.9)
- removed the R5 at (320.5, 137.9)
- removed the R5 at (360.5, 137.9)
- removed the R5 at (364.5, 137.9)
- removed the R5 at (356.5, 137.9)
- removed the R5 at (352.5, 137.9)
- removed the R5 at (368.5, 137.9)
- removed the R5 at (284.5, 137.9)
- removed the R5 at (348.5, 137.9)
- removed the R5 at (332.5, 137.9)
- removed the R5 at (336.5, 137.9)
- removed the R5 at (344.5, 137.9)
- removed the R5 at (340.5, 137.9)
- removed the R5 at (372.5, 137.9)
- removed the R5 at (376.5, 137.9)
- removed the R5 at (300.5, 137.9)
- removed the R5 at (304.5, 137.9)
- removed the R5 at (296.5, 137.9)
- removed the R5 at (292.5, 137.9)
- removed the R5 at (308.5, 137.9)
- removed the R6 at (288.5, 167.9)
- removed the R6 at (328.5, 167.9)
- removed the R6 at (312.5, 167.9)
- removed the R6 at (316.5, 167.9)
- removed the R6 at (324.5, 167.9)
- removed the R6 at (320.5, 167.9)
- removed the R6 at (360.5, 167.9)
- removed the R6 at (364.5, 167.9)
- removed the R6 at (356.5, 167.9)
- removed the R6 at (352.5, 167.9)
- removed the R6 at (368.5, 167.9)
- removed the R6 at (284.5, 167.9)
- removed the R6 at (348.5, 167.9)
- removed the R6 at (332.5, 167.9)
- removed the R6 at (336.5, 167.9)
- removed the R6 at (344.5, 167.9)
- removed the R6 at (340.5, 167.9)
- removed the R6 at (372.5, 167.9)
- removed the R6 at (376.5, 167.9)
- removed the R6 at (300.5, 167.9)
- removed the R6 at (304.5, 167.9)
- removed the R6 at (296.5, 167.9)
- removed the R6 at (292.5, 167.9)
- removed the R6 at (308.5, 167.9)
- added D1: LED, my_parts:MADW__CHIPLED-0805, F.Cu at (262.1, 120.0)
- added D1: LED, my_parts:MADW__CHIPLED-0805, F.Cu at (218.1, 120.0)
- added D1: LED, my_parts:MADW__CHIPLED-0805, F.Cu at (210.1, 120.0)
- added D1: LED, my_parts:MADW__CHIPLED-0805, F.Cu at (206.1, 120.0)
- added D1: LED, my_parts:MADW__CHIPLED-0805, F.Cu at (222.1, 120.0)
- added D1: LED, my_parts:MADW__CHIPLED-0805, F.Cu at (226.1, 120.0)
- added D1: LED, my_parts:MADW__CHIPLED-0805, F.Cu at (234.1, 120.0)
- added D1: LED, my_parts:MADW__CHIPLED-0805, F.Cu at (230.1, 120.0)
- added D1: LED, my_parts:MADW__CHIPLED-0805, F.Cu at (198.1, 120.0)
- added D1: LED, my_parts:MADW__CHIPLED-0805, F.Cu at (202.1, 120.0)
- added D1: LED, my_parts:MADW__CHIPLED-0805, F.Cu at (194.1, 120.0)
- added D1: LED, my_parts:MADW__CHIPLED-0805, F.Cu at (266.1, 120.0)
- added D1: LED, my_parts:MADW__CHIPLED-0805, F.Cu at (190.1, 120.0)
- added D1: LED, my_parts:MADW__CHIPLED-0805, F.Cu at (174.1, 120.0)
- added D1: LED, my_parts:MADW__CHIPLED-0805, F.Cu at (178.1, 120.0)
- added D1: LED, my_parts:MADW__CHIPLED-0805, F.Cu at (186.1, 120.0)
- added D1: LED, my_parts:MADW__CHIPLED-0805, F.Cu at (182.1, 120.0)
- added D1: LED, my_parts:MADW__CHIPLED-0805, F.Cu at (258.1, 120.0)
- added D1: LED, my_parts:MADW__CHIPLED-0805, F.Cu at (254.1, 120.0)
- added D1: LED, my_parts:MADW__CHIPLED-0805, F.Cu at (238.1, 120.0)
- added D1: LED, my_parts:MADW__CHIPLED-0805, F.Cu at (242.1, 120.0)
- added D1: LED, my_parts:MADW__CHIPLED-0805, F.Cu at (250.1, 120.0)
- added D1: LED, my_parts:MADW__CHIPLED-0805, F.Cu at (246.1, 120.0)
- added D1: LED, my_parts:MADW__CHIPLED-0805, F.Cu at (214.1, 120.0)
- added D10: LED, my_parts:MADW__CHIPLED-0805, B.Cu at (262.1, 60.0)
- added D10: LED, my_parts:MADW__CHIPLED-0805, B.Cu at (218.1, 60.0)
- added D10: LED, my_parts:MADW__CHIPLED-0805, B.Cu at (210.1, 60.0)
- added D10: LED, my_parts:MADW__CHIPLED-0805, B.Cu at (206.1, 60.0)
- added D10: LED, my_parts:MADW__CHIPLED-0805, B.Cu at (222.1, 60.0)
- added D10: LED, my_parts:MADW__CHIPLED-0805, B.Cu at (226.1, 60.0)
- added D10: LED, my_parts:MADW__CHIPLED-0805, B.Cu at (234.1, 60.0)
- added D10: LED, my_parts:MADW__CHIPLED-0805, B.Cu at (230.1, 60.0)
- added D10: LED, my_parts:MADW__CHIPLED-0805, B.Cu at (198.1, 60.0)
- added D10: LED, my_parts:MADW__CHIPLED-0805, B.Cu at (202.1, 60.0)
- added D10: LED, my_parts:MADW__CHIPLED-0805, B.Cu at (194.1, 60.0)
- added D10: LED, my_parts:MADW__CHIPLED-0805, B.Cu at (266.1, 60.0)
- added D10: LED, my_parts:MADW__CHIPLED-0805, B.Cu at (190.1, 60.0)
- added D10: LED, my_parts:MADW__CHIPLED-0805, B.Cu at (174.1, 60.0)
- added D10: LED, my_parts:MADW__CHIPLED-0805, B.Cu at (178.1, 60.0)
- added D10: LED, my_parts:MADW__CHIPLED-0805, B.Cu at (186.1, 60.0)
- added D10: LED, my_parts:MADW__CHIPLED-0805, B.Cu at (182.1, 60.0)
- added D10: LED, my_parts:MADW__CHIPLED-0805, B.Cu at (258.1, 60.0)
- added D10: LED, my_parts:MADW__CHIPLED-0805, B.Cu at (254.1, 60.0)
- added D10: LED, my_parts:MADW__CHIPLED-0805, B.Cu at (238.1, 60.0)
- added D10: LED, my_parts:MADW__CHIPLED-0805, B.Cu at (242.1, 60.0)
- added D10: LED, my_parts:MADW__CHIPLED-0805, B.Cu at (250.1, 60.0)
- added D10: LED, my_parts:MADW__CHIPLED-0805, B.Cu at (246.1, 60.0)
- added D10: LED, my_parts:MADW__CHIPLED-0805, B.Cu at (214.1, 60.0)
- added D11: LED, my_parts:MADW__CHIPLED-0805, B.Cu at (262.1, 70.0)
- added D11: LED, my_parts:MADW__CHIPLED-0805, B.Cu at (218.1, 70.0)
- added D11: LED, my_parts:MADW__CHIPLED-0805, B.Cu at (210.1, 70.0)
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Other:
- board text added: "2014 V0.20.b"
- board text removed: "2014 V0.20.a"
